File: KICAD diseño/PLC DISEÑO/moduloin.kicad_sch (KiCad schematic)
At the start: 8 parts

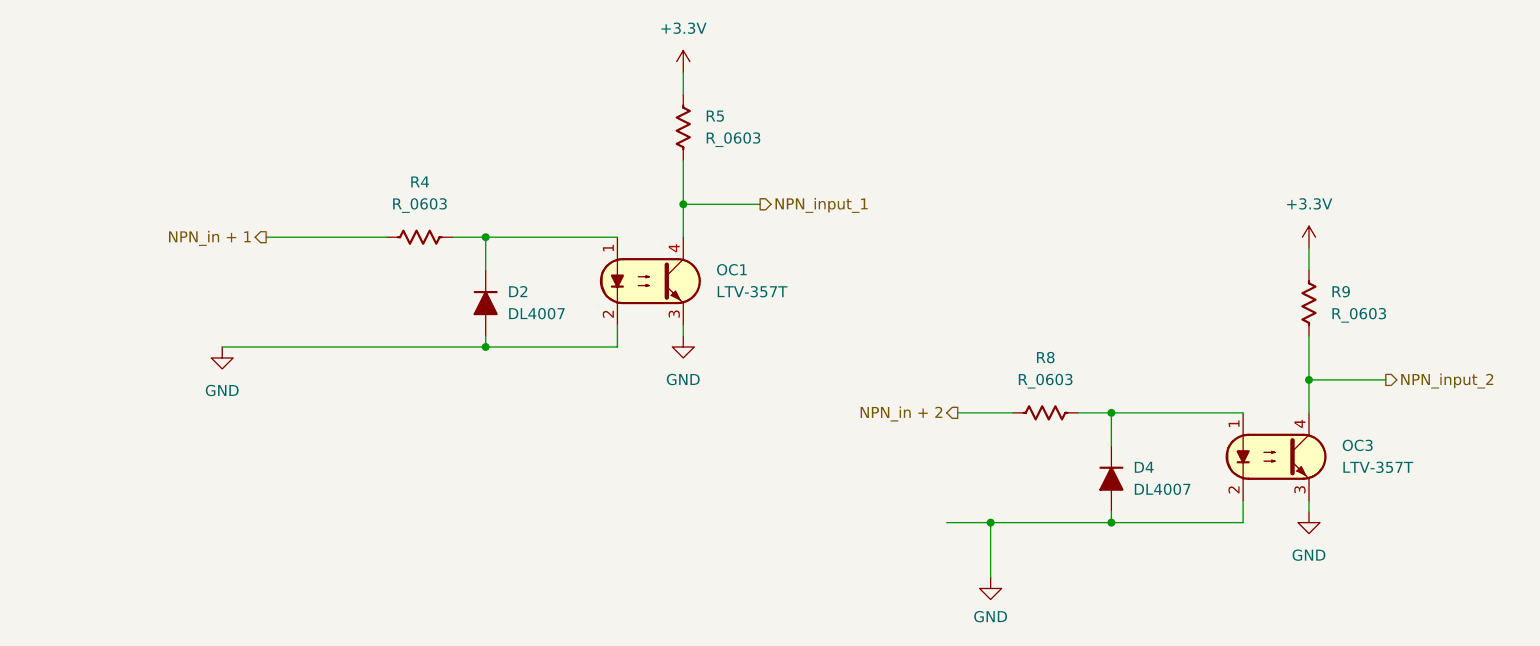
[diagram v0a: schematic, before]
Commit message: Nirvara actualization :>
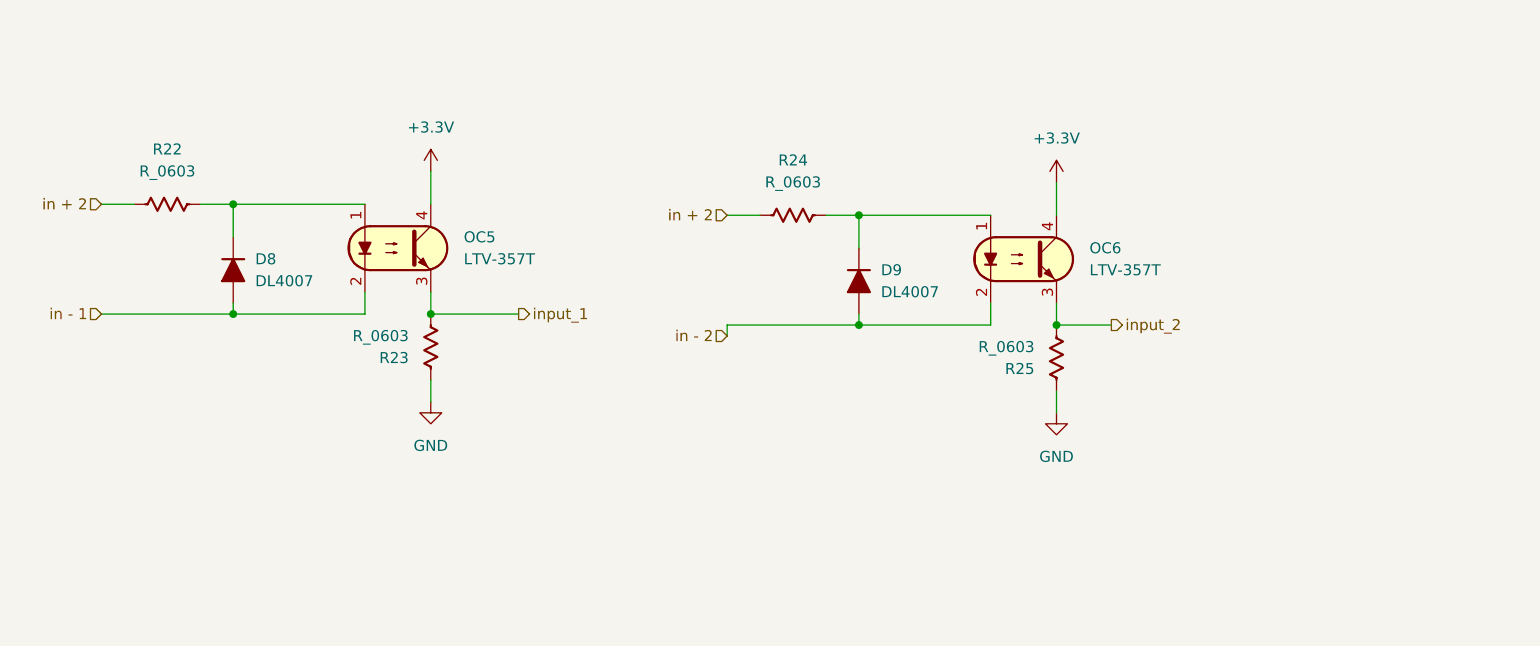
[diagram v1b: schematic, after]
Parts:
- removed D2, D4: DL4007, PCM_Diode_SMD_AKL:D_MELF, symbol PCM_Diode_AKL:DL4007
- removed OC1, OC3: LTV-357T, PCM_Package_SO_AKL:SO-4_4.4x3.9mm_P2.54mm, symbol PCM_Optocoupler_AKL:LTV-357T
- removed R4, R5, R8, R9: R_0603, PCM_Resistor_SMD_AKL:R_0603_1608Metric, symbol PCM_Resistor_US_AKL:R_0603
- added D8, D9: DL4007, PCM_Diode_SMD_AKL:D_MELF, symbol PCM_Diode_AKL:DL4007
- added OC5, OC6: LTV-357T, PCM_Package_SO_AKL:SO-4_4.4x3.9mm_P2.54mm, symbol PCM_Optocoupler_AKL:LTV-357T
- added R22, R23, R24, R25: R_0603, PCM_Resistor_SMD_AKL:R_0603_1608Metric, symbol PCM_Resistor_US_AKL:R_0603
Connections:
- net +3.3V: now also OC5.4, OC6.4
- net GND: now also R23.1, R25.1
- new net: D9.1 (K), OC6.1, R24.2
- new net: D8.1 (K), OC5.1, R22.2
- new net in + 2: R22.1, R24.1
- new net in - 1: D8.2 (A), OC5.2
- new net in - 2: D9.2 (A), OC6.2
- new net input_1: OC5.3, R23.2
- new net input_2: OC6.3, R25.2
